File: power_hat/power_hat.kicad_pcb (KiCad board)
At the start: 4 copper layers, 50 x 120 mm, 71 parts, among them IC1 TPS259830LNRGER, IC2 INA238AQDGSRQ1, J1 XT30PW-M/Terminal block, J13 502585-0570, J14 502585-0570, J2 XT30PW-M/Terminal block, J3 XT30PW-M/Terminal block, J4 XT30PW-M/Terminal block, J5 Conn_01x02_Pin, J6 XT30PW-M/Terminal block, J7 Conn_01x02_Pin, J8 XT30PW-M/Terminal block, Q1 CSD18540Q5B, Q2 SIR5607DP-T1-UE3, Q3 SIR5607DP-T1-UE3, U17 ADM1270ARQZ

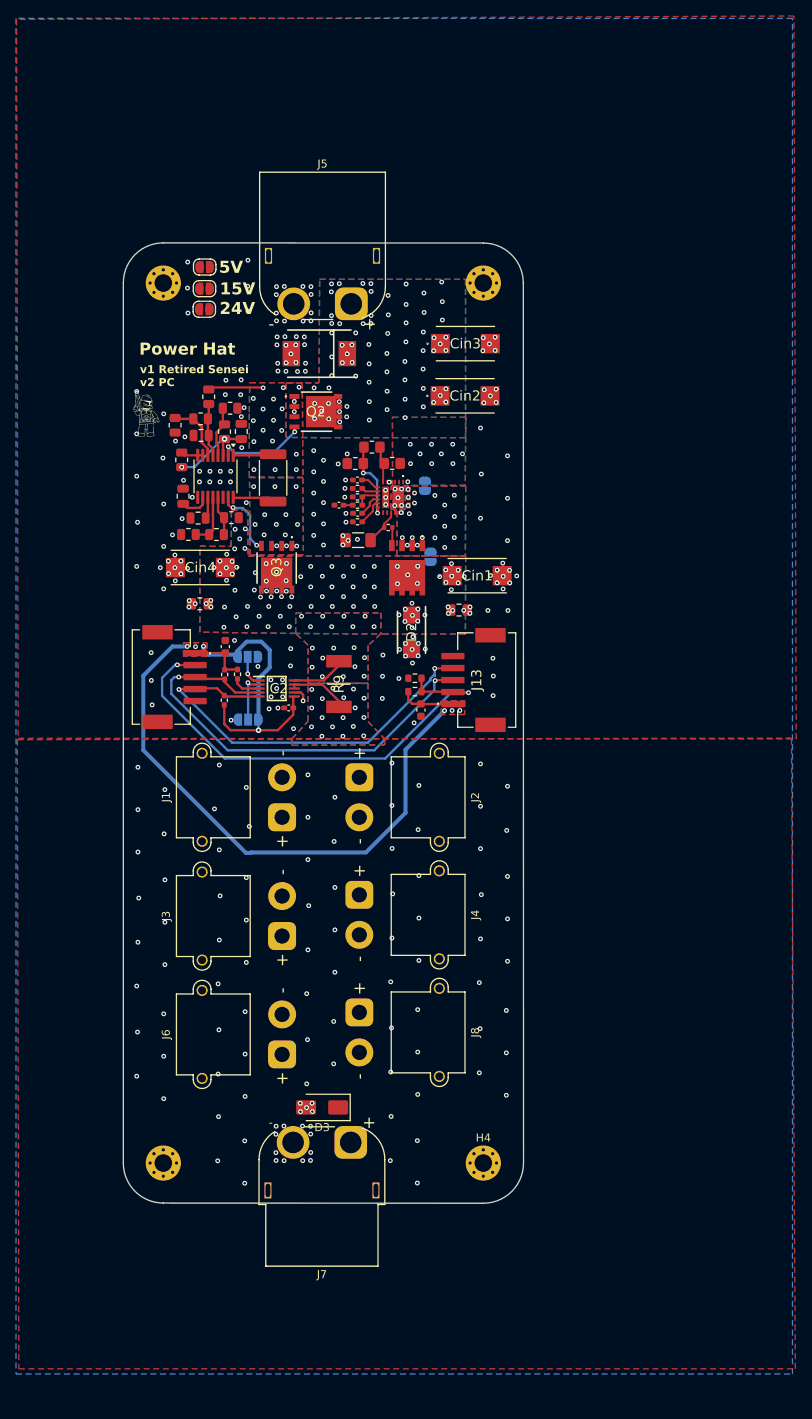
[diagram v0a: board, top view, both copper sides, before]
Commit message: Already bought but forgot to commit
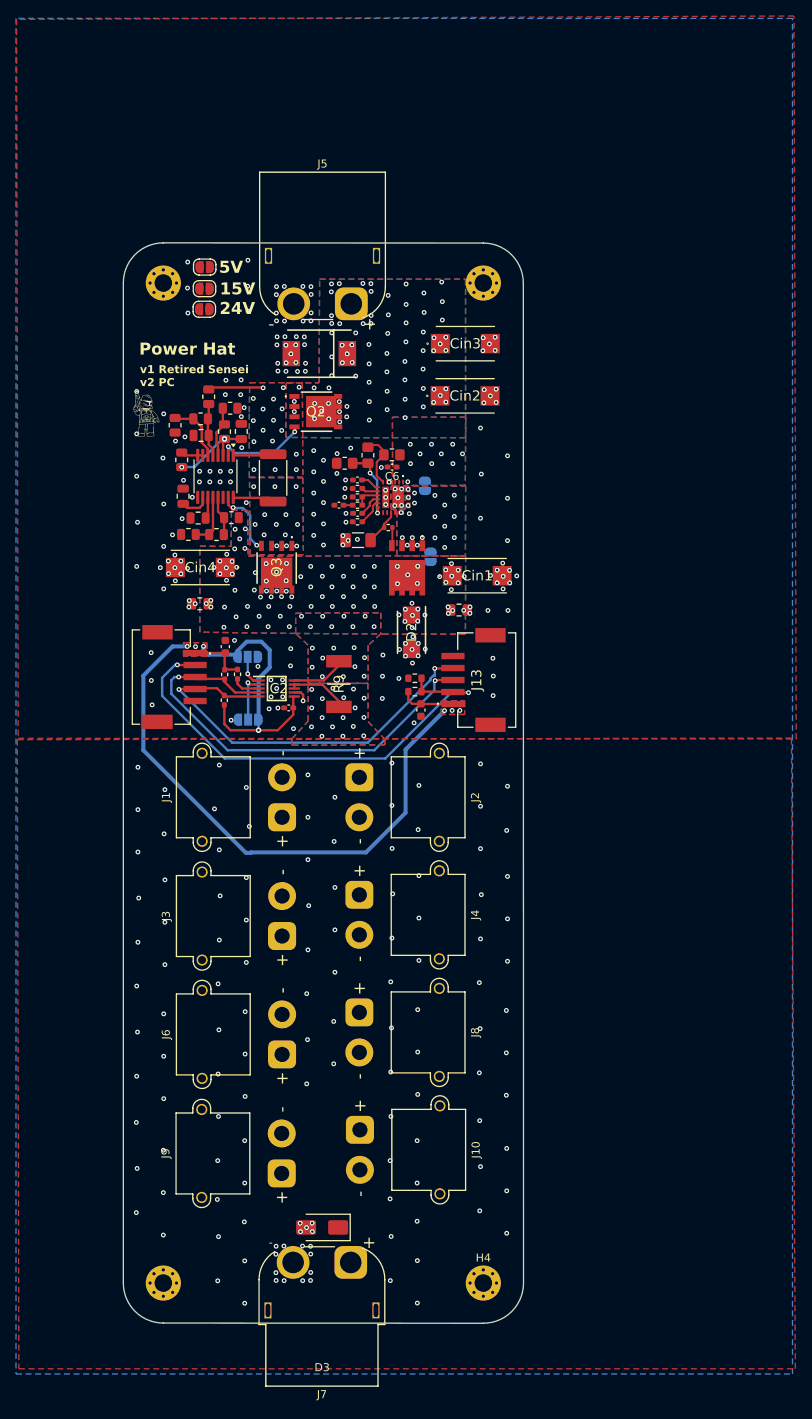
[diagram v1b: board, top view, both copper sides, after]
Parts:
- added C6: 0.1uF, Capacitor_SMD:C_0402_1005Metric_Pad0.74x0.62mm_HandSolder, F.Cu at (92.0, 76.7)
- added J10: XT30PW-M/Terminal block, Corrected_XT60:AMASS_XT30PW-M_1x02_P2.50mm_Horizontal, F.Cu at (88.0, 164.5)
- added J9: XT30PW-M/Terminal block, Corrected_XT60:AMASS_XT30PW-M_1x02_P2.50mm_Horizontal, F.Cu at (78.2, 159.9)
- moved D3 15.0 mm to (83.2, 171.7)
- moved H2 15.0 mm to (63.4, 178.6)
- moved H4 15.0 mm to (103.4, 178.6)
- moved J7 15.0 mm to (79.6, 176.1)
- moved R3 1.33 mm to (86.1, 76.2)
- moved R2 1.13 mm to (89.0, 75.2), turned to -90 degrees
- moved R1 1.07 mm to (92.0, 75.1)
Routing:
- net Net-(IC1-EN/UVLO): track 4.64 -> 7.02 mm
- net Net-(IC1-OVLO): track 10.2 -> 9.35 mm
- net GND: vias 273 -> 299
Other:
- board size 50 x 120 mm -> 50 x 135 mm
